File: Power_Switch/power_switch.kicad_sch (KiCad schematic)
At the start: 6 parts, among them J1 Conn_01x03_Pin, SW1 SW_SPDT

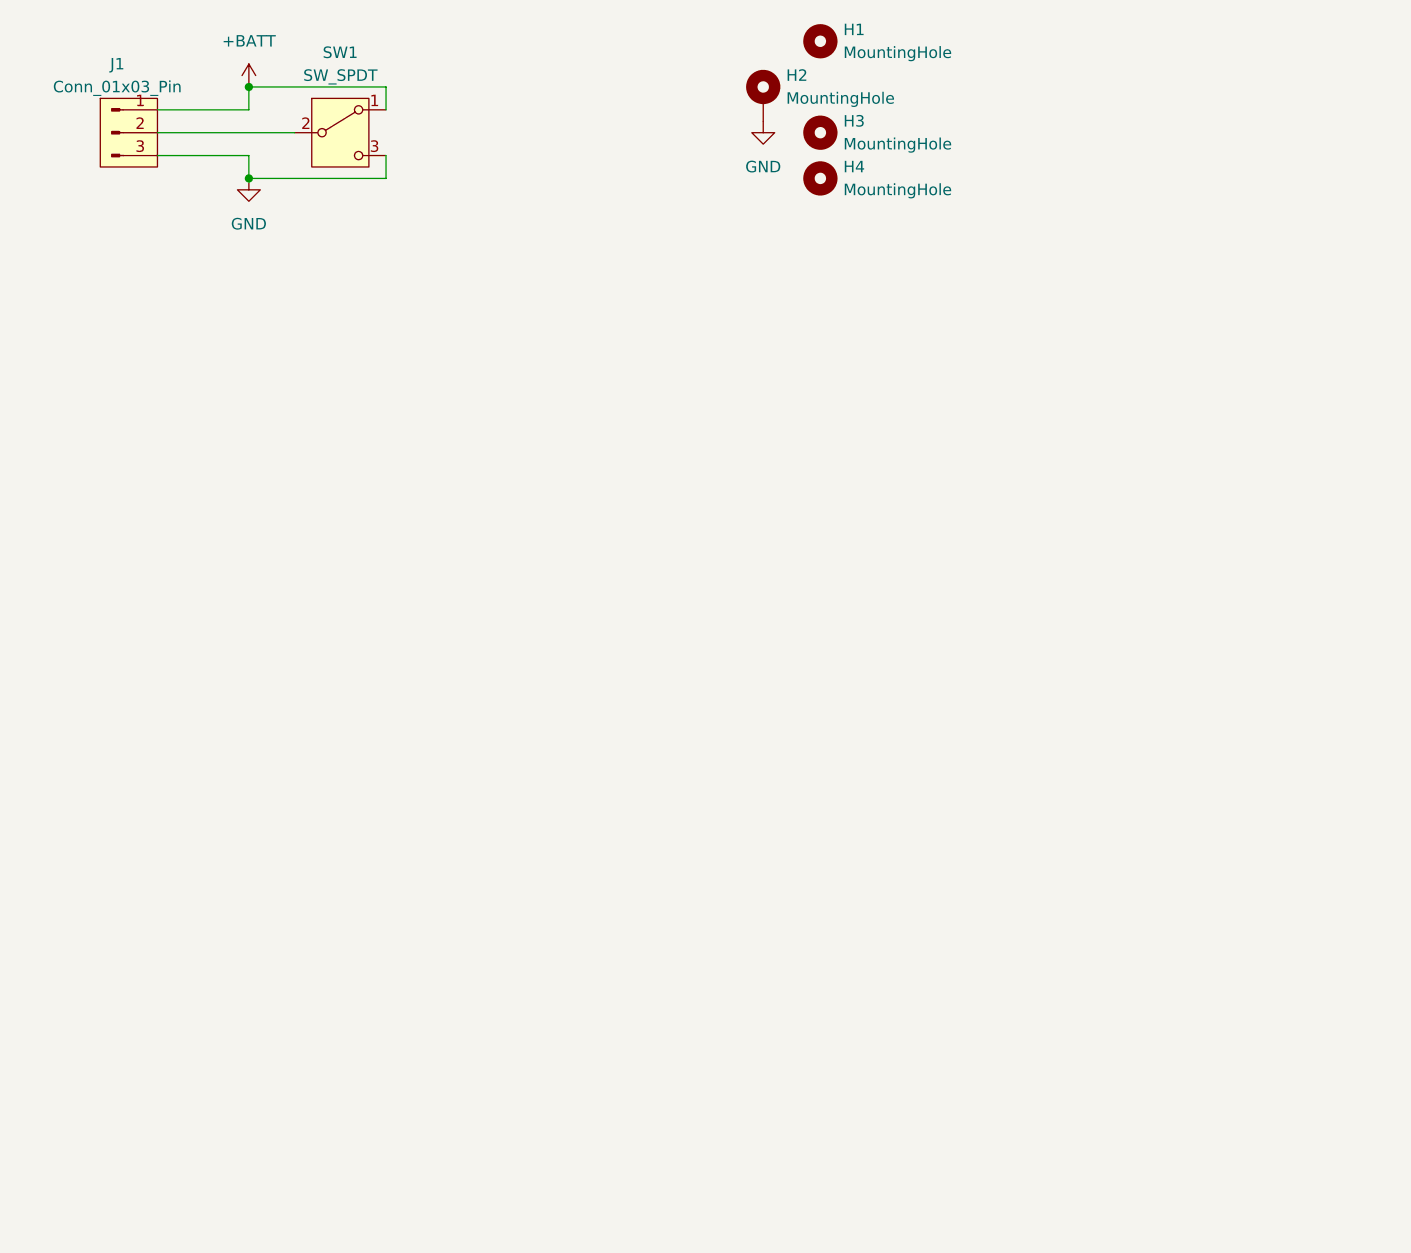
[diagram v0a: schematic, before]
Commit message: Orginizing and small work done
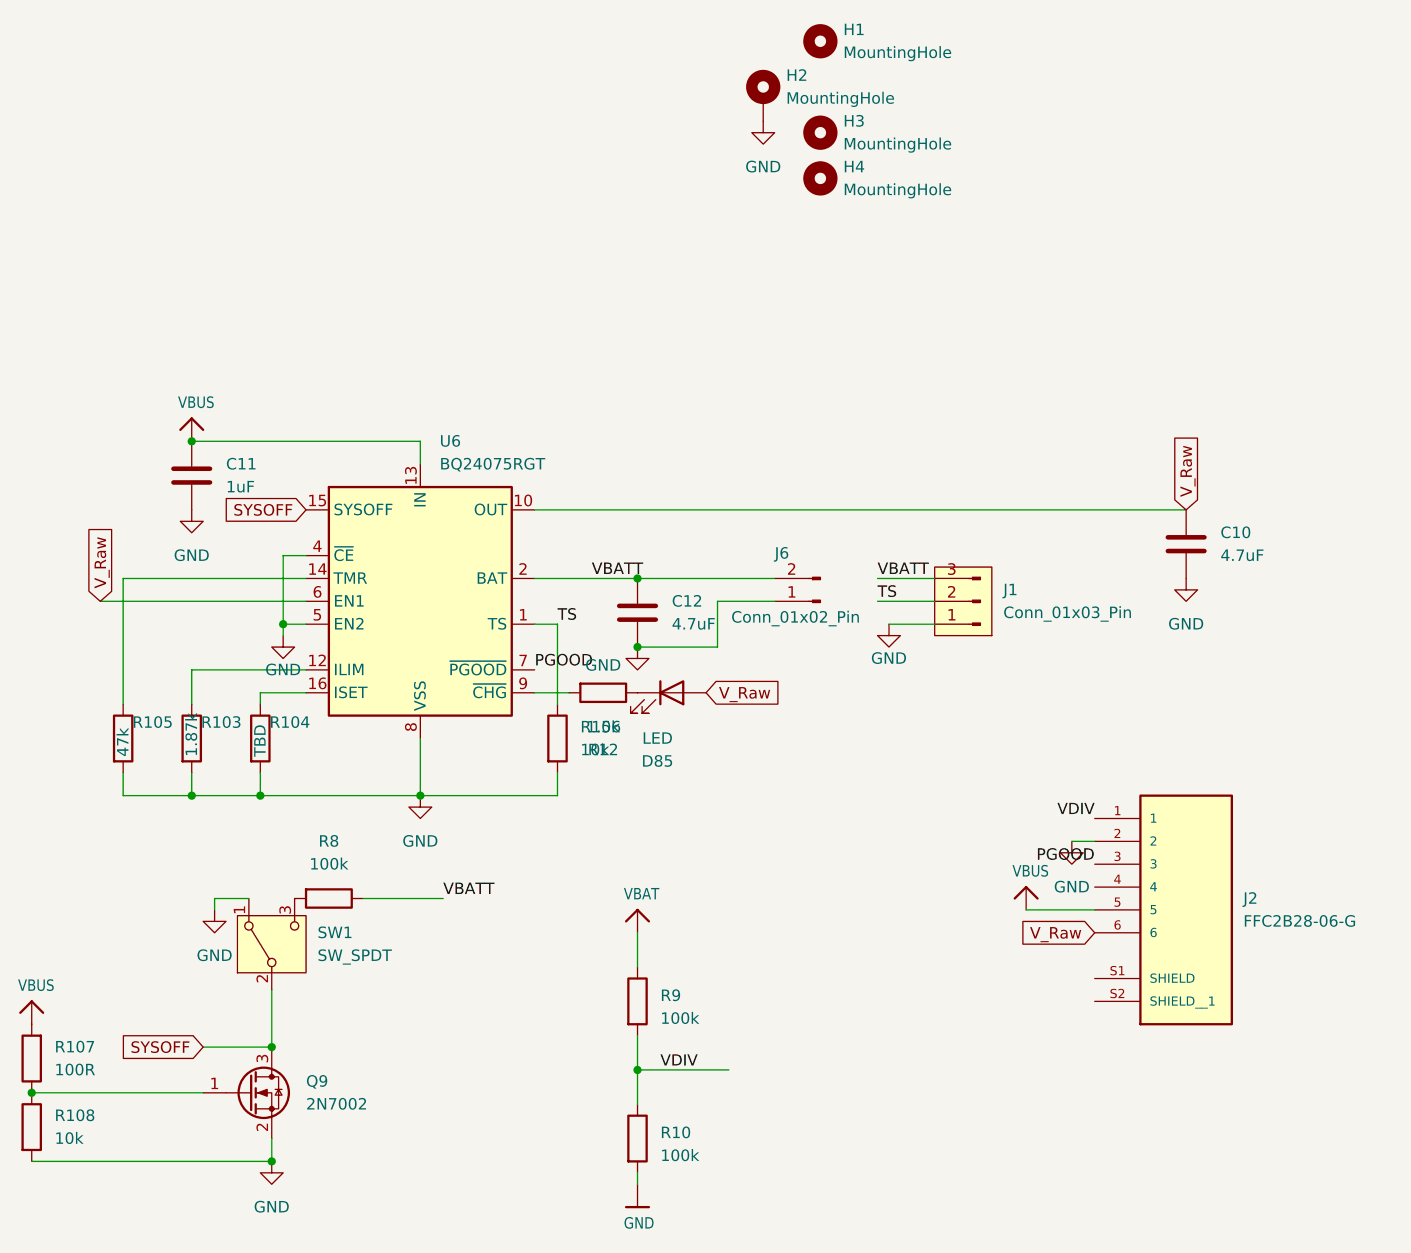
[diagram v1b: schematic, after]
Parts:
- added C10, C12: 4.7uF, Capacitor_SMD:C_0402_1005Metric, symbol Device:C
- added C11: 1uF, Capacitor_SMD:C_0402_1005Metric, symbol Device:C
- added D85: LED, JohnDeereLibrary:LED_WURTH_155060AS75300, symbol Device:LED
- added J2: FFC2B28-06-G, GCT:GCT_FFC2B28-06-G, symbol FFC2B28-06-G:FFC2B28-06-G
- added J6: Conn_01x02_Pin, Connector_PinSocket_2.54mm:PinSocket_1x02_P2.54mm_Vertical, symbol Connector:Conn_01x02_Pin
- added Q9: 2N7002, Package_TO_SOT_SMD:SOT-23, symbol Transistor_FET:2N7002
- added R10, R8, R9: 100k, Resistor_SMD:R_0402_1005Metric, symbol Device:R
- added R103: 1.87k, Resistor_SMD:R_0402_1005Metric, symbol Device:R
- added R104: TBD, Resistor_SMD:R_0402_1005Metric, symbol Device:R
- added R105: 47k, Resistor_SMD:R_0402_1005Metric, symbol Device:R
- added R106, R108: 10k, Resistor_SMD:R_0402_1005Metric, symbol Device:R
- added R107: 100R, Resistor_SMD:R_0402_1005Metric, symbol Device:R
- added R12: 1.5k, Resistor_SMD:R_0402_1005Metric, symbol Device:R
- added U6: BQ24075RGT, Package_DFN_QFN:VQFN-16-1EP_3x3mm_P0.5mm_EP1.6x1.6mm, symbol Battery_Management:BQ24075RGT
- SW1: footprint JohnDeereLibrary:ET01M3D1SAPE -> JohnDeereLibrary:ET01MD1CBE
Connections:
- net +BATT is gone; now on net GND: J1.1 (Pin_1), SW1.1 (A)
- net GND: now also C10.2, C11.2, C12.2, J2.2, J6.1 (Pin_1), Q9.2 (S), R10.2, R103.2, R104.2, R105.2, R106.2, R108.2, U6.17 (VSS), U6.4 (~{CE}), U6.5 (EN2), U6.8 (VSS); no longer J1.3 (Pin_3), SW1.3 (C)
- net SYSOFF: now reaches SW1.2 (B)
- net SYSOFF: now also Q9.3 (D), U6.15 (SYSOFF); no longer J1.2 (Pin_2)
- new net: R8.2, SW1.3 (C)
- new net: R104.1, U6.16 (ISET)
- new net: Q9.1 (G), R107.1, R108.1
- new net: R105.1, U6.14 (TMR)
- new net: D85.1 (K), R12.1
- new net: R12.2, U6.9 (~{CHG})
- new net: R103.1, U6.12 (ILIM)
- new net PGOOD: J2.3, U6.7 (~{PGOOD})
- new net TS: J1.2 (Pin_2), R106.1, U6.1 (TS)
- new net VBAT: R9.1
- new net VBATT: C12.1, J1.3 (Pin_3), J6.2 (Pin_2), R8.1, U6.2 (BAT), U6.3 (BAT)
- new net VBUS: C11.1, J2.5, R107.2, U6.13 (IN)
- new net VDIV: J2.1, R10.1, R9.2
- new net V_Raw: C10.1, D85.2 (A), J2.6, U6.10 (OUT), U6.11 (OUT), U6.6 (EN1)
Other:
- moved on the sheet: J1, SW1
